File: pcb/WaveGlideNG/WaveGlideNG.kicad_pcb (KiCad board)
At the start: 2 copper layers, 72 x 70.6 mm, 23 parts

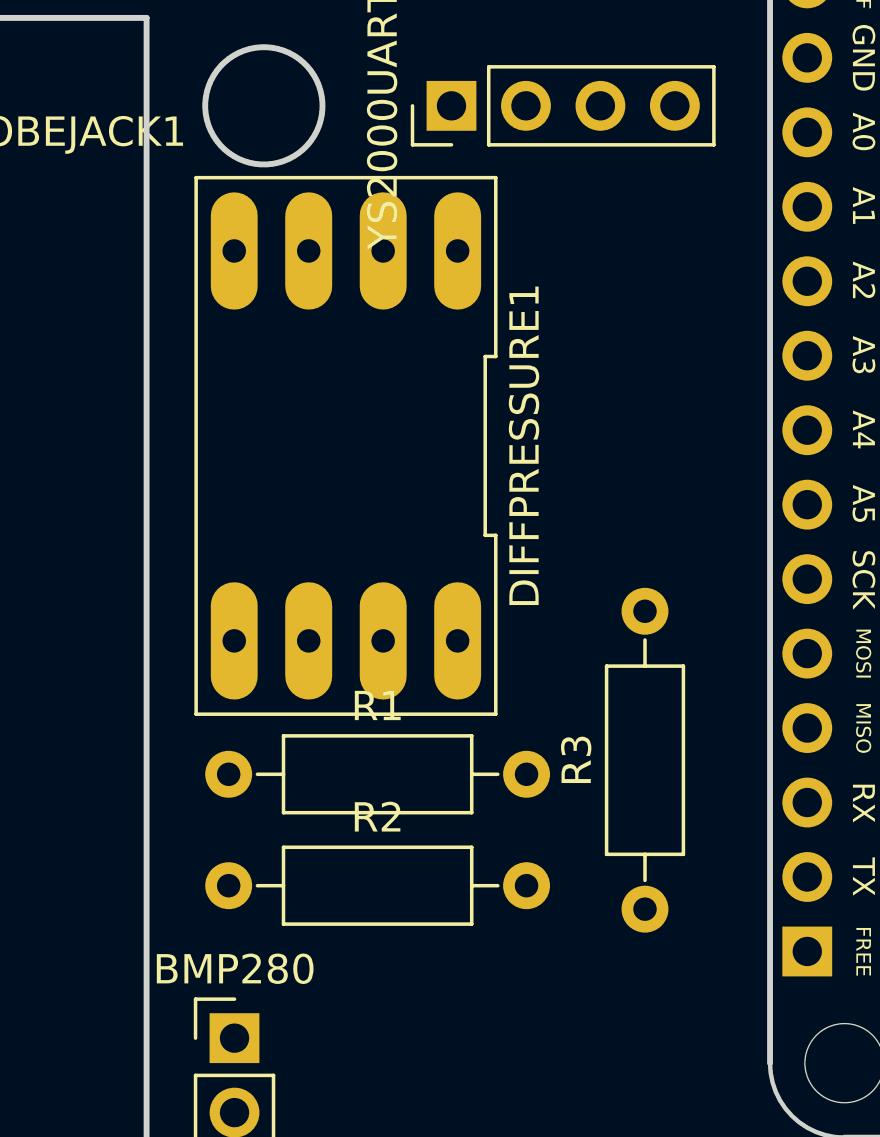
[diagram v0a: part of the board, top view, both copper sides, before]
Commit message: footprints
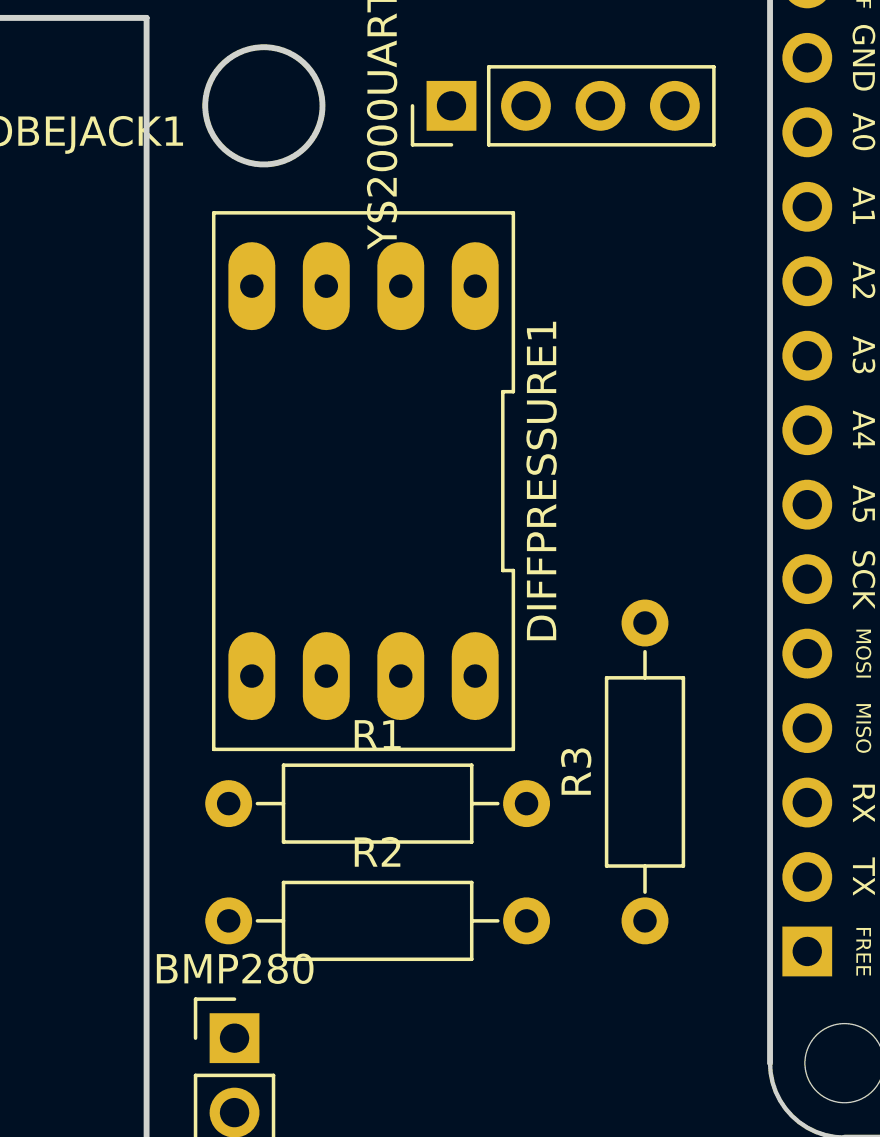
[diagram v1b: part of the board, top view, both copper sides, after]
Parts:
- moved DIFFPRESSURE1 1.34 mm to (102.6, 104.0)
- moved R2 1.20 mm to (98.0, 119.0)
- moved R1 1.00 mm to (98.0, 115.0)
- moved R3 0.40 mm to (112.2, 119.0)
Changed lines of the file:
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@@
     (pad 8 thru_hole circle (at 0 0) (size 2.4 2.4) (drill 1.4) (layers *.Cu *.Mask))
-  )
-  (module WaveGlideNG:DIFFPRESS (layer F.Cu)
-    (at 102 102.8 180)
-    (descr SSCMRRN001PDAA3)
-    (fp_text reference DIFFPRESSURE1 (at -6.11 0 90) (layer F.SilkS)
-      (effects (font (size 1 1) (thickness 0.15)))
-    )
-    (fp_text value PressSensor (at 0 0) (layer F.Fab)
-      (effects (font (size 1 1) (thickness 0.15)))
-    )
-    (fp_line (start -5.11 9.15) (end 5.109999 9.15) (layer F.SilkS) (width 0.12))
-    (fp_line (start 5.109999 9.15) (end 5.11 -9.15) (layer F.SilkS) (width 0.12))
-    (fp_line (start 5.11 -9.15) (end -5.109999 -9.15) (layer F.SilkS) (width 0.12))
-    (fp_line (start -5.109999 -9.15) (end -5.11 -3.05) (layer F.SilkS) (width 0.12))
-    (fp_line (start -5.11 -3.05) (end -4.75 -3.05) (layer F.SilkS) (width 0.12))
-    (fp_line (start -4.75 -3.05) (end -4.75 3.049999) (layer F.SilkS) (width 0.12))
-    (fp_line (start -4.75 3.049999) (end -5.11 3.049999) (layer F.SilkS) (width 0.12))
-    (fp_line (start -5.11 3.049999) (end -5.11 9.15) (layer F.SilkS) (width 0.12))
-    (fp_line (start -4.86 -8.9) (end 4.86 -8.9) (layer F.CrtYd) (width 0.05))
-    (fp_line (start 4.86 -8.9) (end 4.86 8.9) (layer F.CrtYd) (width 0.05))
-    (fp_line (start 4.86 8.9) (end -4.86 8.9) (layer F.CrtYd) (width 0.05))
-    (fp_line (start -4.86 8.9) (end -4.86 -8.9) (layer F.CrtYd) (width 0.05))
-    (pad 8 thru_hole oval (at -3.81 -6.65 180) (size 1.6 4) (drill 0.8) (layers *.Cu *.Mask))
-    (pad 1 thru_hole oval (at -3.81 6.65 180) (size 1.6 4) (drill 0.8) (layers *.Cu *.Mask))
-    (pad 7 thru_hole oval (at -1.27 -6.65 180) (size 1.6 4) (drill 0.8) (layers *.Cu *.Mask))
-    (pad 2 thru_hole oval (at -1.27 6.65 180) (size 1.6 4) (drill 0.8) (layers *.Cu *.Mask)
-      (net 7 +3V3))
-    (pad 6 thru_hole oval (at 1.27 -6.65 180) (size 1.6 4) (drill 0.8) (layers *.Cu *.Mask))
-    (pad 3 thru_hole oval (at 1.27 6.65 180) (size 1.6 4) (drill 0.8) (layers *.Cu *.Mask)
-      (net 10 IN_DIFFPRES))
-    (pad 5 thru_hole oval (at 3.81 -6.65 180) (size 1.6 4) (drill 0.8) (layers *.Cu *.Mask))
-    (pad 4 thru_hole oval (at 3.81 6.65 180) (size 1.6 4) (drill 0.8) (layers *.Cu *.Mask)
-      (net 6 GND))
   )
   (module WaveGlideNG:PIEZO (layer F.Cu)
@@
   )
   (module Resistors_ThroughHole:R_Axial_DIN0207_L6.3mm_D2.5mm_P10.16mm_Horizontal (layer F.Cu)
-    (at 98 114)
+    (at 98 115)
     (descr "Resistor, Axial_DIN0207 series, Axial, Horizontal, pin pitch=10.16mm, 0.25W = 1/4W, length*diameter=6.3*2.5mm^2, http://cdn-reichelt.de/documents/datenblatt/B400/1_4W%23YAG.pdf")
     (tags "Resistor Axial_DIN0207 series Axial Horizontal pin pitch 10.16mm 0.25W = 1/4W length 6.3mm diameter 2.5mm")
@@
   )
   (module Resistors_ThroughHole:R_Axial_DIN0207_L6.3mm_D2.5mm_P10.16mm_Horizontal (layer F.Cu)
-    (at 98 117.8)
+    (at 98 119)
     (descr "Resistor, Axial_DIN0207 series, Axial, Horizontal, pin pitch=10.16mm, 0.25W = 1/4W, length*diameter=6.3*2.5mm^2, http://cdn-reichelt.de/documents/datenblatt/B400/1_4W%23YAG.pdf")
     (tags "Resistor Axial_DIN0207 series Axial Horizontal pin pitch 10.16mm 0.25W = 1/4W length 6.3mm diameter 2.5mm")
@@
   )
   (module Resistors_ThroughHole:R_Axial_DIN0207_L6.3mm_D2.5mm_P10.16mm_Horizontal (layer F.Cu)
-    (at 112.2 118.6 90)
+    (at 112.2 119 90)
     (descr "Resistor, Axial_DIN0207 series, Axial, Horizontal, pin pitch=10.16mm, 0.25W = 1/4W, length*diameter=6.3*2.5mm^2, http://cdn-reichelt.de/documents/datenblatt/B400/1_4W%23YAG.pdf")
     (tags "Resistor Axial_DIN0207 series Axial Horizontal pin pitch 10.16mm 0.25W = 1/4W length 6.3mm diameter 2.5mm")
@@
       (net 6 GND))
   )
+  (module WaveGlideNG:DIFFPRESS (layer F.Cu)
+    (at 102.6 104 180)
+    (descr SSCMRRN001PDAA3)
+    (fp_text reference DIFFPRESSURE1 (at -6.11 0 90) (layer F.SilkS)
+      (effects (font (size 1 1) (thickness 0.15)))
+    )
+    (fp_text value PressSensor (at 0 0) (layer F.Fab)
+      (effects (font (size 1 1) (thickness 0.15)))
+    )
+    (fp_line (start -5.11 9.15) (end 5.109999 9.15) (layer F.SilkS) (width 0.12))
+    (fp_line (start 5.109999 9.15) (end 5.11 -9.15) (layer F.SilkS) (width 0.12))
+    (fp_line (start 5.11 -9.15) (end -5.109999 -9.15) (layer F.SilkS) (width 0.12))
+    (fp_line (start -5.109999 -9.15) (end -5.11 -3.05) (layer F.SilkS) (width 0.12))
+    (fp_line (start -5.11 -3.05) (end -4.75 -3.05) (layer F.SilkS) (width 0.12))
+    (fp_line (start -4.75 -3.05) (end -4.75 3.049999) (layer F.SilkS) (width 0.12))
+    (fp_line (start -4.75 3.049999) (end -5.11 3.049999) (layer F.SilkS) (width 0.12))
+    (fp_line (start -5.11 3.049999) (end -5.11 9.15) (layer F.SilkS) (width 0.12))
+    (fp_line (start -4.86 -8.9) (end 4.86 -8.9) (layer F.CrtYd) (width 0.05))
+    (fp_line (start 4.86 -8.9) (end 4.86 8.9) (layer F.CrtYd) (width 0.05))
+    (fp_line (start 4.86 8.9) (end -4.86 8.9) (layer F.CrtYd) (width 0.05))
+    (fp_line (start -4.86 8.9) (end -4.86 -8.9) (layer F.CrtYd) (width 0.05))
+    (pad 8 thru_hole oval (at -3.81 -6.65 180) (size 1.6 3) (drill 0.8) (layers *.Cu *.Mask))
+    (pad 1 thru_hole oval (at -3.81 6.65 180) (size 1.6 3) (drill 0.8) (layers *.Cu *.Mask))
+    (pad 7 thru_hole oval (at -1.27 -6.65 180) (size 1.6 3) (drill 0.8) (layers *.Cu *.Mask))
+    (pad 2 thru_hole oval (at -1.27 6.65 180) (size 1.6 3) (drill 0.8) (layers *.Cu *.Mask)
+      (net 7 +3V3))
+    (pad 6 thru_hole oval (at 1.27 -6.65 180) (size 1.6 3) (drill 0.8) (layers *.Cu *.Mask))
+    (pad 3 thru_hole oval (at 1.27 6.65 180) (size 1.6 3) (drill 0.8) (layers *.Cu *.Mask)
+      (net 10 IN_DIFFPRES))
+    (pad 5 thru_hole oval (at 3.81 -6.65 180) (size 1.6 3) (drill 0.8) (layers *.Cu *.Mask))
+    (pad 4 thru_hole oval (at 3.81 6.65 180) (size 1.6 3) (drill 0.8) (layers *.Cu *.Mask)
+      (net 6 GND))
+  )
